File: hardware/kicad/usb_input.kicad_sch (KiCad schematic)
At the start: 19 parts, among them J1 MC-107DMS, Q1 2N7002, U1 TPS70933DBVR, U2 TUSB320LAIRWBR, U3 SN74LVC1G02DBVR

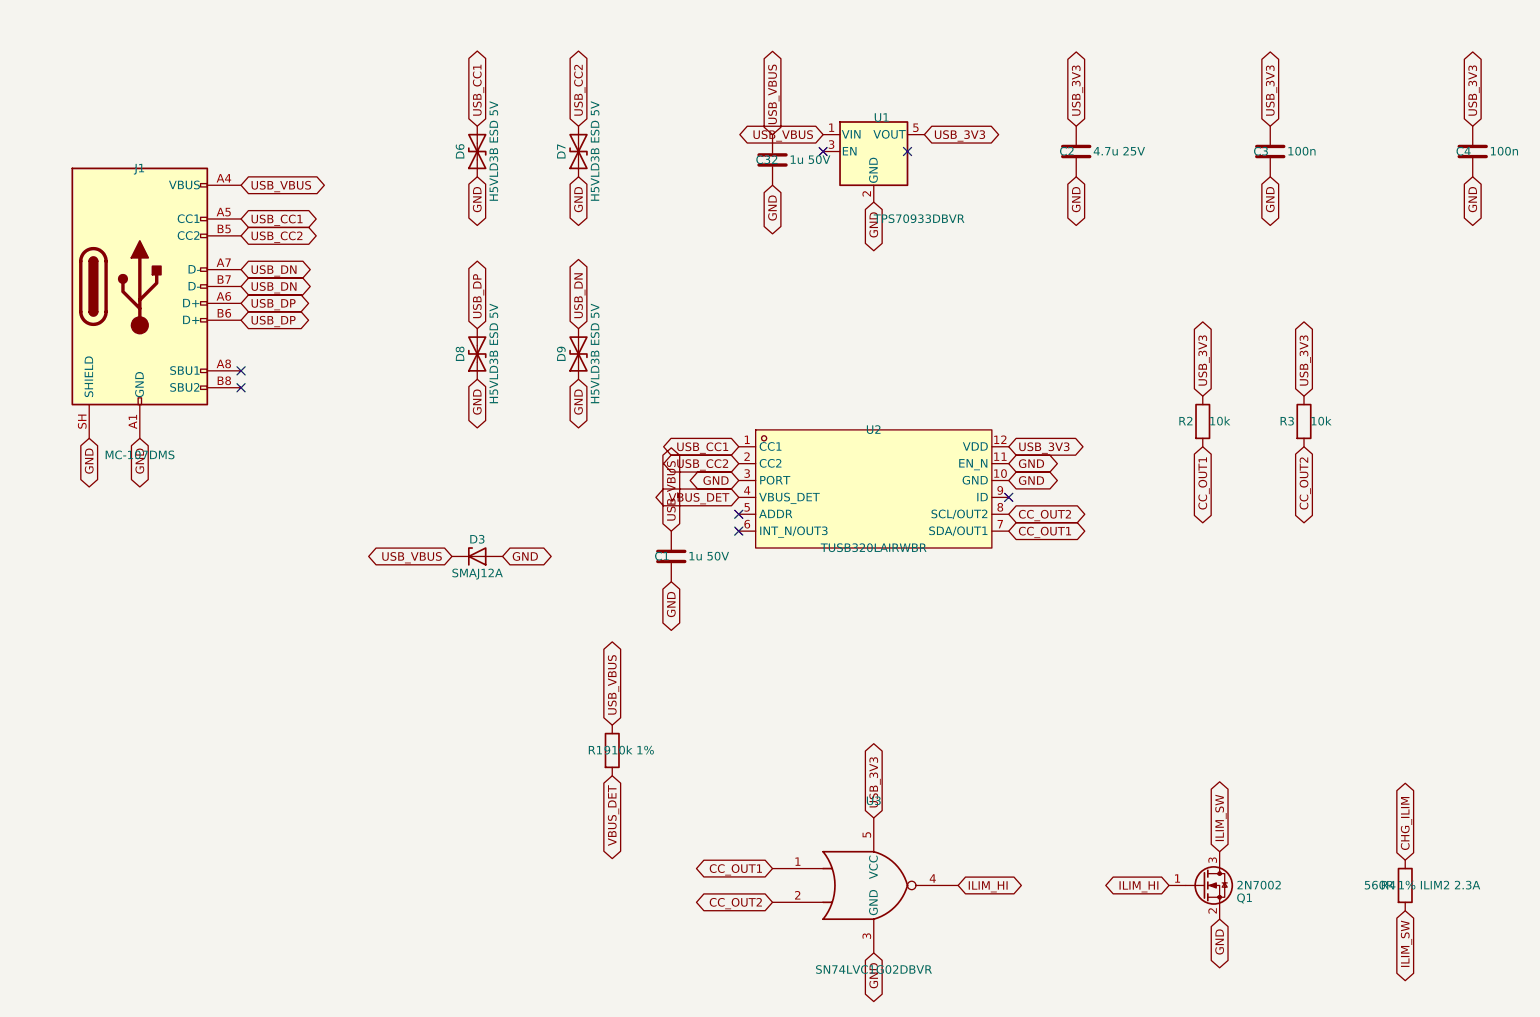
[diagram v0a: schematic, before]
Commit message: Revise charger
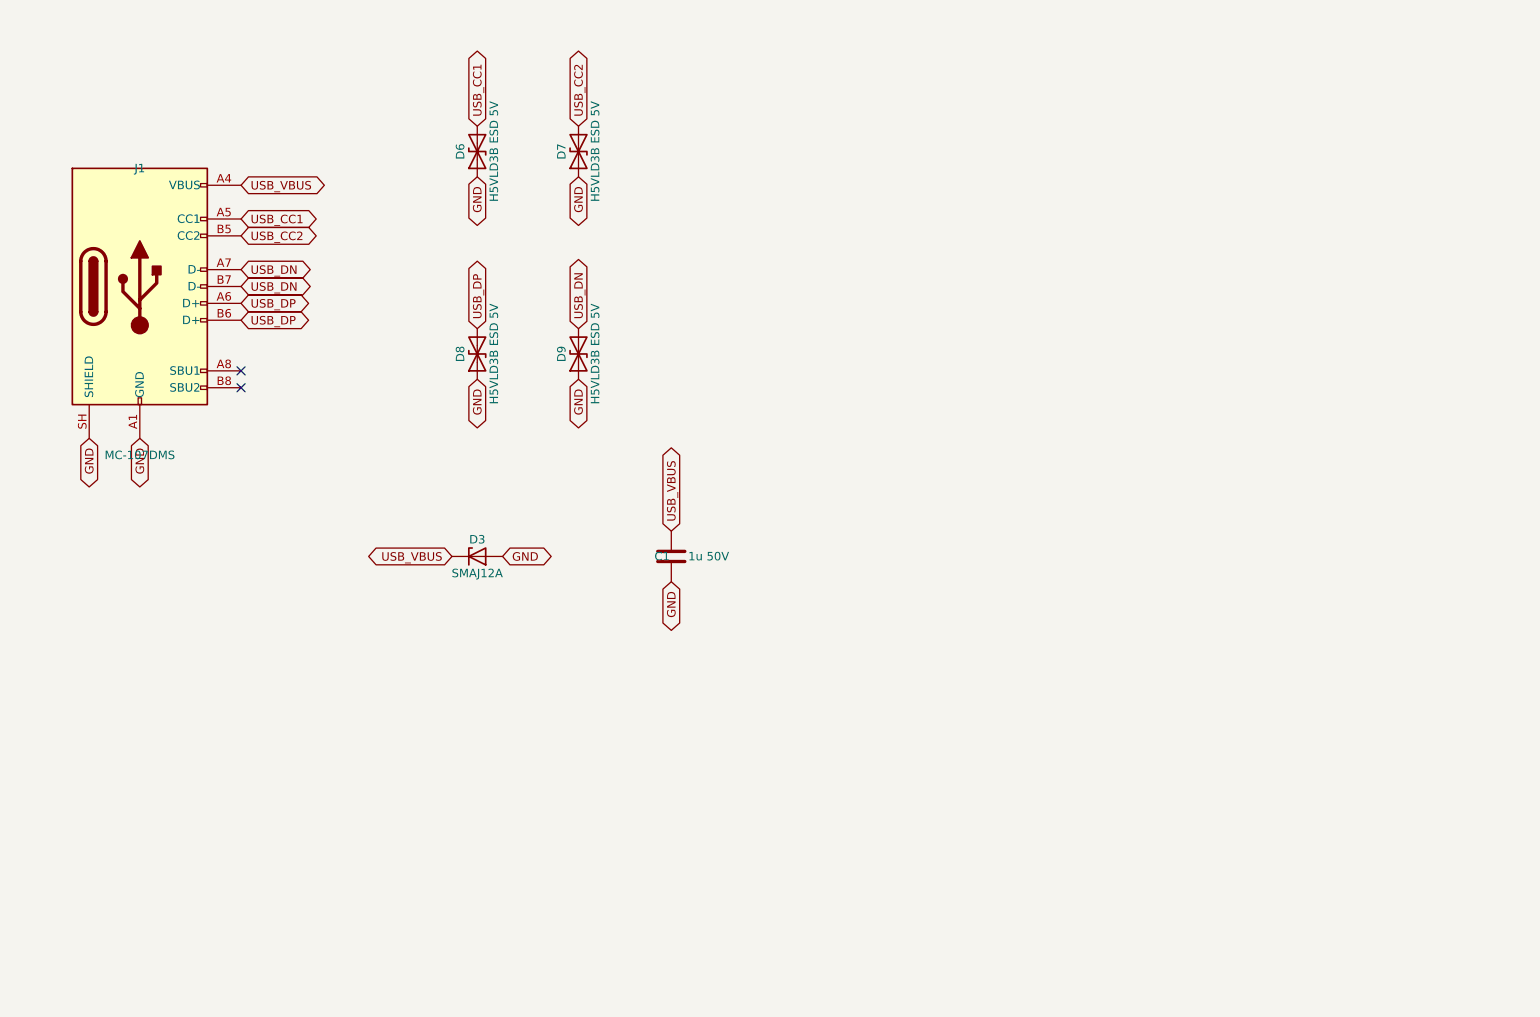
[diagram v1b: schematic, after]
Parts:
- removed C2: 4.7u 25V, Capacitor_SMD:C_0805_2012Metric, symbol Device:C
- removed C3, C4: 100n, Capacitor_SMD:C_0603_1608Metric, symbol Device:C
- removed C32: 1u 50V, Capacitor_SMD:C_0603_1608Metric, symbol Device:C
- removed Q1: 2N7002, Package_TO_SOT_SMD:SOT-23, symbol Transistor_FET:2N7002
- removed R1: 910k 1%, Resistor_SMD:R_0603_1608Metric, symbol Device:R
- removed R2, R3: 10k, Resistor_SMD:R_0603_1608Metric, symbol Device:R
- removed R4: 560R 1% ILIM2 2.3A, Resistor_SMD:R_0603_1608Metric, symbol Device:R
- removed U1: TPS70933DBVR, Package_TO_SOT_SMD:SOT-23-5, symbol Regulator_Linear:AP2112K-3.3
- removed U2: TUSB320LAIRWBR, Package_DFN_QFN:Texas_X2QFN-12_1.6x1.6mm_P0.4mm, symbol carrier:TUSB320LAIRWBR
- removed U3: SN74LVC1G02DBVR, Package_TO_SOT_SMD:SOT-23-5, symbol 74xGxx:74LVC1G02
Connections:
- no-connect marks 7 -> 2

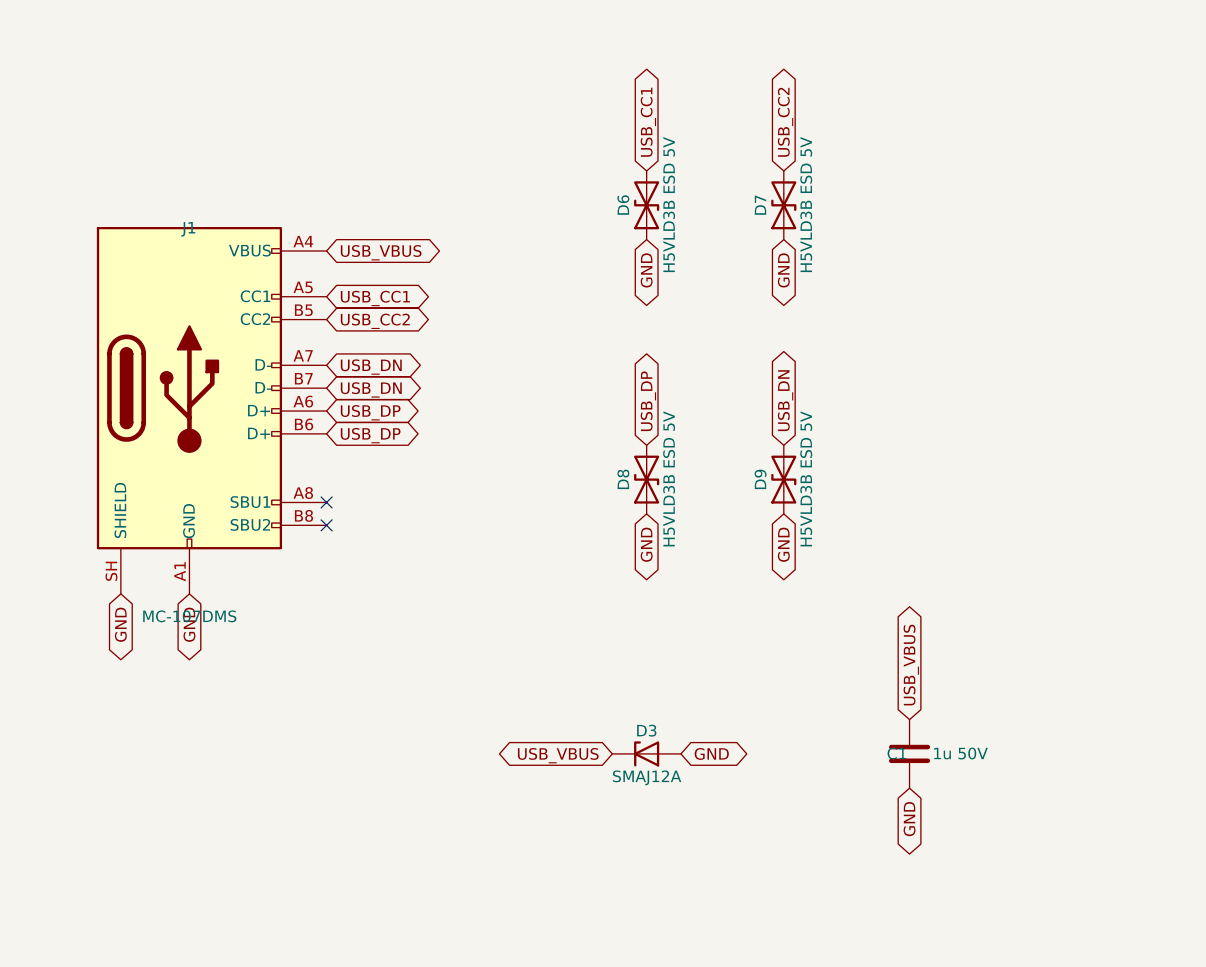
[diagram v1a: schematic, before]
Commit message: Cleanups
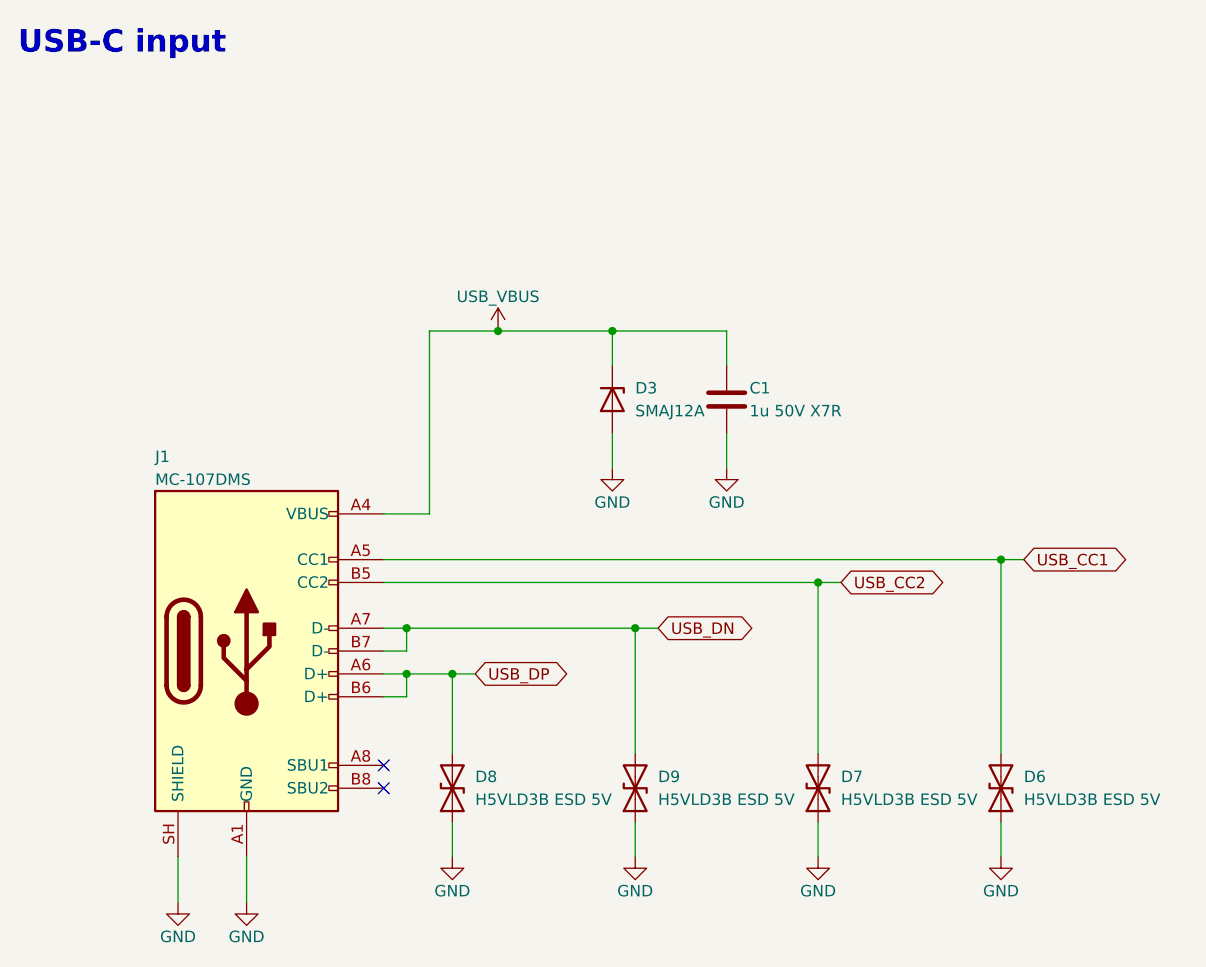
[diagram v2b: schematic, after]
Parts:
- C1: value 1u 50V -> 1u 50V X7R; LCSC C15849 -> C105174
- D6, D7, D8, D9: MPN (none) -> H5VLD3B; Manufacturer (none) -> Zhuhai Hongjiacheng (R+O)
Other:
- note added: "USB-C input"
- title: (none) -> USB input
- moved on the sheet: C1, D3, D6, D7, D8, D9, J1
